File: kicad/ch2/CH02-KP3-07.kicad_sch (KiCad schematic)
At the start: 5 parts

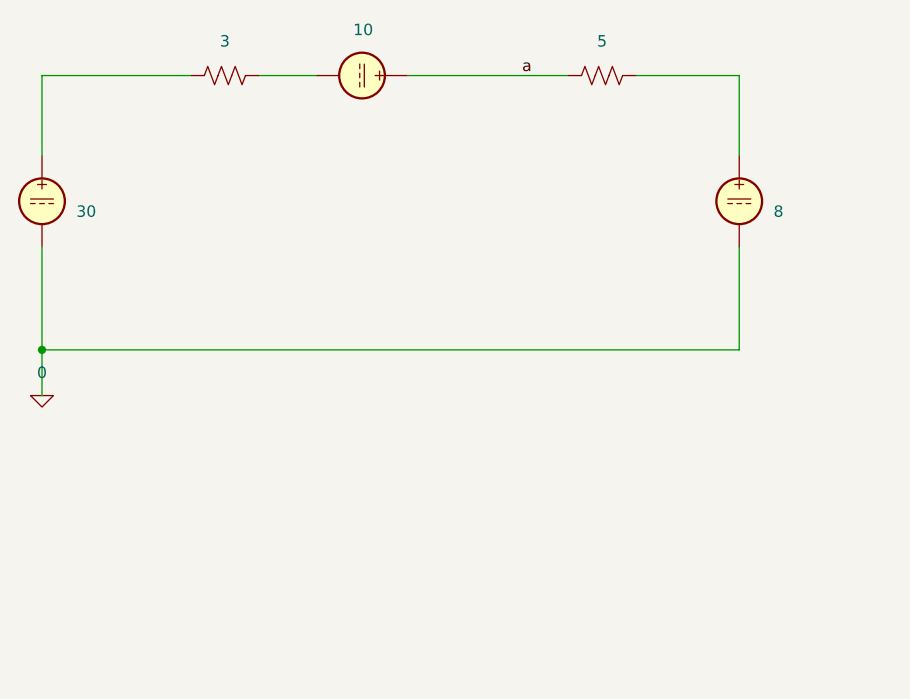
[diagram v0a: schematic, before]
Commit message: regular
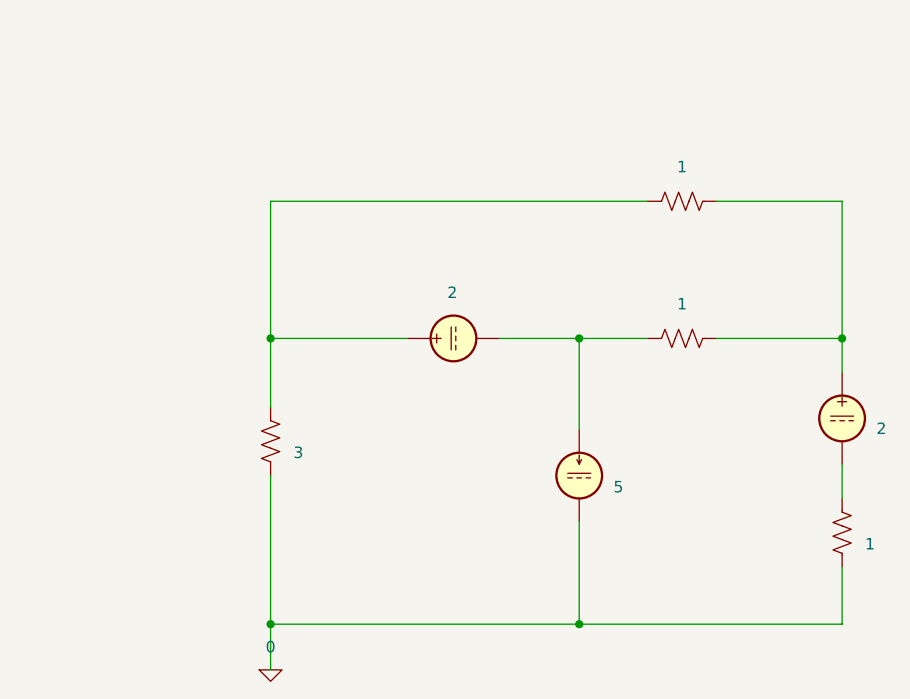
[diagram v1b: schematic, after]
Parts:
- removed R4: 3, symbol Device:R_US
- removed R5: 5, symbol Device:R_US
- removed V3: 30, symbol Simulation_SPICE:VDC
- removed V4: 10, symbol Simulation_SPICE:VDC
- removed V5: 8, symbol Simulation_SPICE:VDC
- added I4: 5, symbol Simulation_SPICE:IDC
- added R20: 3, symbol Device:R_US
- added R21, R22, R23: 1, symbol Device:R_US
- added V10, V11: 2, symbol Simulation_SPICE:VDC
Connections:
- net 0: now also I4.2, R20.2, R21.2
- new net: R22.1, R23.2, V10.1
- new net: R20.1, R22.2, V11.1
- new net: I4.1, R23.1, V11.2
- new net: R21.1, V10.2
